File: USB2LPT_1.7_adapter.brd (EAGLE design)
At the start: 43.4 x 49.5 mm, 27 parts

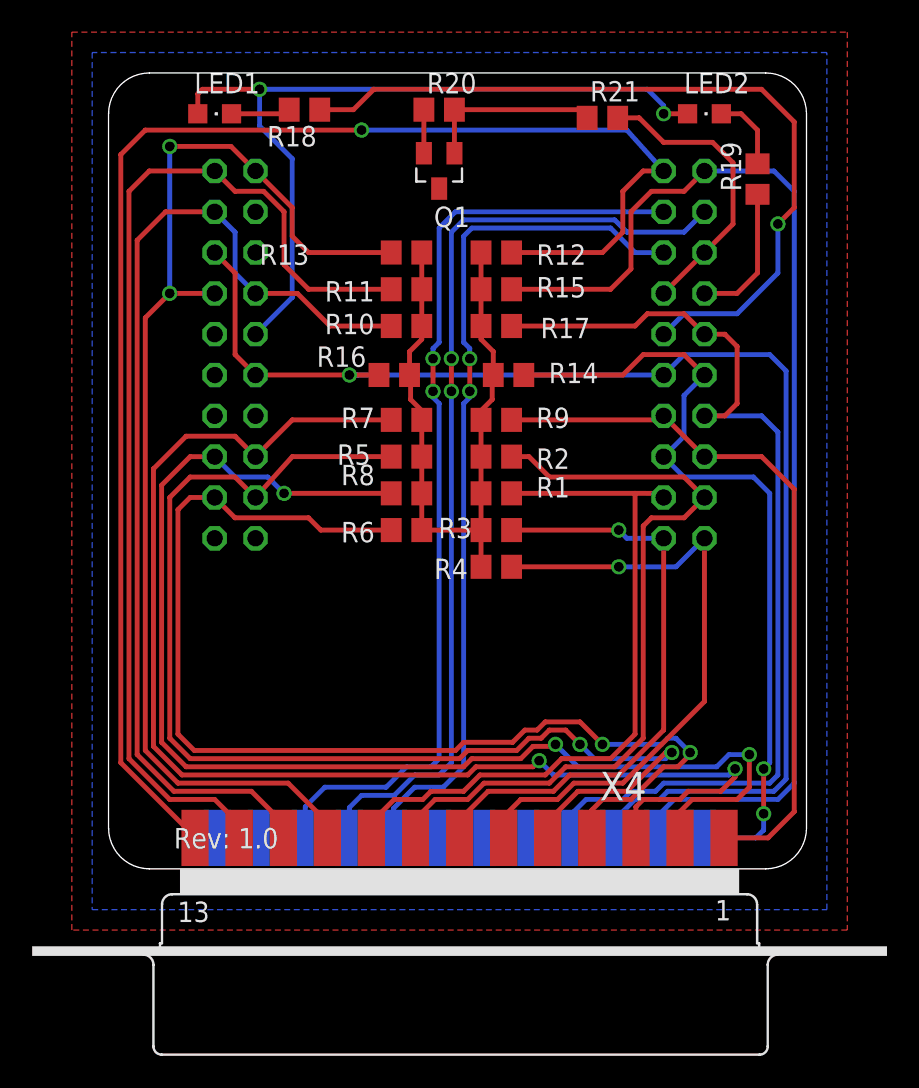
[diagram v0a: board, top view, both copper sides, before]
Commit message: idem
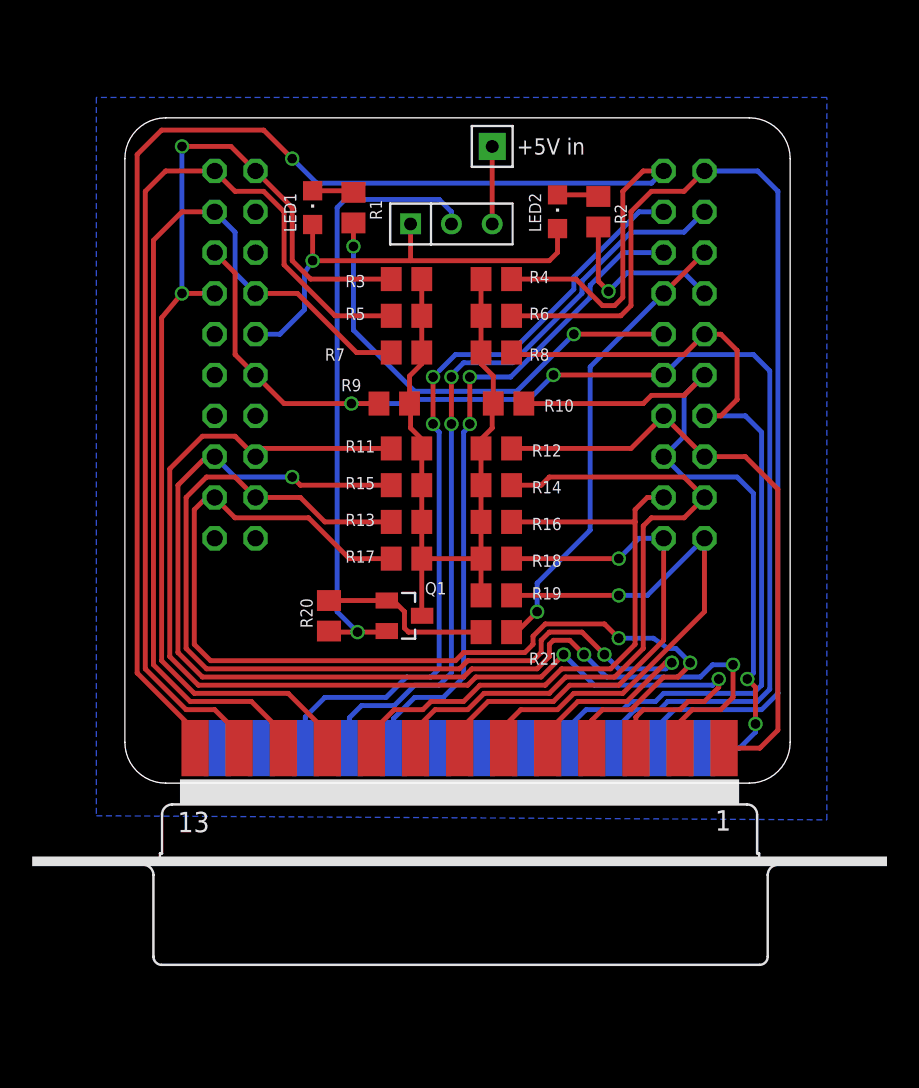
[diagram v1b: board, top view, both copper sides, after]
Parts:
- removed X4: (no value), con-subd:F25D
- added +5V: CON_HEADER_1X01-PTH_08_17, dp_devices:M1X2_08_17
- added J1: CON_HEADER_1X03-PTH, dp_devices:M1X3
- added U$1: (no value), dp_devices:JUMP3_DESC_LEFT
- added U$5: (no value), dp_devices:JUMP3_DESC_RIGHT
- added X101: (no value), con-lstb:MA10-2
- R1, R2: value 4K7 -> 470
- R12, R6, R8: value 4K7 -> 2K2
- R15, R16, R17: value 2K2 -> 4K7
- R18, R19: value 470 -> 4K7
- X1: device con-lstb:MA10-2 -> con-subd:F25D
- moved X1 33.6 mm to (19.1, 1.47), flipped to the top, turned to 180 degrees
- moved R21 32.7 mm to (21.3, 14.7)
- moved R20 32.2 mm to (10.9, 15.7), turned to 90 degrees
- moved R19 30.6 mm to (21.3, 17.0), turned to 180 degrees
- moved R18 30.4 mm to (21.3, 19.3)
- moved Q1 27.8 mm to (15.6, 15.7), turned to 270 degrees
- moved R1 19.9 mm to (12.4, 41.1), turned to 90 degrees
- moved R4 17.9 mm to (21.3, 36.7)
- moved R13 16.8 mm to (15.7, 21.6)
- moved R3 16.6 mm to (15.7, 36.7), turned to 0 degrees
- moved R2 16.5 mm to (27.7, 40.9), turned to 90 degrees
- moved R17 15.5 mm to (15.7, 19.3), turned to 0 degrees
- moved R6 14.5 mm to (21.3, 34.4), turned to 180 degrees
- moved R15 13.4 mm to (15.7, 23.9), turned to 0 degrees
- moved R12 12.2 mm to (21.3, 26.2)
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- renumbered X2 to X100
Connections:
- new net 5V_PAD: +5V.1, J1.3
- new net VSELECT: J1.2, Q1.2, R20.1
- net +3V3: now also J1.1, X101.12, X101.2; no longer Q1.2, R20.1, X1.12, X1.2
- net CTL0: now also R12.1, X1.1; no longer R9.1, X4.1
- net CTL1: now also R10.1, X1.14; no longer R14.1, X4.14
- net CTL2: now also R8.1, X1.17; no longer R17.1, X4.17
- net GND: now also X1.19, X1.20, X1.24, X1.25, X101.1, X101.11, X101.16, X101.18, X101.9; no longer X1.1, X1.11, X1.16, X1.9, X4.18, X4.19, X4.20, X4.24, X4.25
- net IFCLK: now also R9.1, X1.16, X101.10, X101.15; no longer R16.1, X1.10, X1.15, X4.16
- net N$5: now also R1.2; no longer R18.2
- net N$6: now also R2.2; no longer R19.2
- net PA4: now also R1.1; no longer R18.1
- net PA5: now also R2.1; no longer R19.1
- net PB0: now also R15.1, X1.2, X101.5; no longer R8.1, X1.5, X4.2
- net PB1: now also R11.1, X1.3, X101.6; no longer R7.1, X1.6, X4.3
- net PB2: now also R17.1, X1.4, X101.3; no longer R6.1, X1.3, X4.4
- net PB3: now also R13.1, X1.5, X101.4; no longer R5.1, X1.4, X4.5
- net PB4: now also R19.1, X1.6; no longer R4.1, X4.6
- net PB5: now also R18.1, X1.7; no longer R3.1, X4.7
- net PB6: now also R14.1, X1.8; no longer R2.1, X4.8
- net PB7: now also R16.1, X1.9; no longer R1.1, X4.9
- net PD0: now also X1.21; no longer X4.21
- net PD1: now also X1.22; no longer X4.22
- net PD2: now also X1.23; no longer X4.23
- net PD3: now also R6.1, X1.15; no longer R15.1, X4.15
- net PD4: now also R4.1, X1.13; no longer R12.1, X4.13
- net PD5: now also R5.1, X1.12, X101.19; no longer R11.1, X1.19, X4.12
- net PD6: now also R3.1, X1.10, X101.13, X101.20; no longer R13.1, X1.13, X1.20, X4.10
- net PD7: now also R7.1, X1.11, X101.14, X101.17; no longer R10.1, X1.14, X1.17, X4.11
- net PULL-UPS: now also R18.2, R19.2; no longer R1.2, R2.2
- net SCL: now also X101.7; no longer X1.7
- net SDA: now also X101.8; no longer X1.8
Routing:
- net VSELECT: track 0.00 -> 39.4 mm, vias 0 -> 1
- net +3V3: track 52.5 -> 28.4 mm, vias 2 -> 1
- net PA4: track 49.5 -> 29.0 mm, vias 1 -> 2
- net PD0: track 53.9 -> 41.8 mm
- net PD1: track 59.3 -> 48.3 mm
- net PD2: track 60.7 -> 49.8 mm
- net PA6: track 18.3 -> 28.8 mm, vias 0 -> 1
- net PB1: track 82.0 -> 72.5 mm
- net PB0: track 79.9 -> 71.2 mm
- net CTL2: track 62.8 -> 54.6 mm
- net CTL1: track 51.3 -> 43.8 mm
- net PB3: track 74.9 -> 67.6 mm
- net PD5: track 66.5 -> 59.6 mm
- net PD7: track 64.8 -> 57.9 mm
- net PD6: track 72.7 -> 66.0 mm
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- removed copper zone on layer 1, net GND
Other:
- board size 43.4 x 49.5 mm -> 41.4 x 41.4 mm
- board text added: "+3.3V IOs"
- board text added: "+5V IOs"
- board text added: "+5V in"
- board text added: "1"
- board text added: "13"
- board text added: "14"
- board text added: "20"
- board text added: "25"
- board text added: "Connect to host board +5Vdc source"
- board text removed: "Rev: 1.0"
